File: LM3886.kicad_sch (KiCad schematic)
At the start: 1 part, among them U1 LM3886

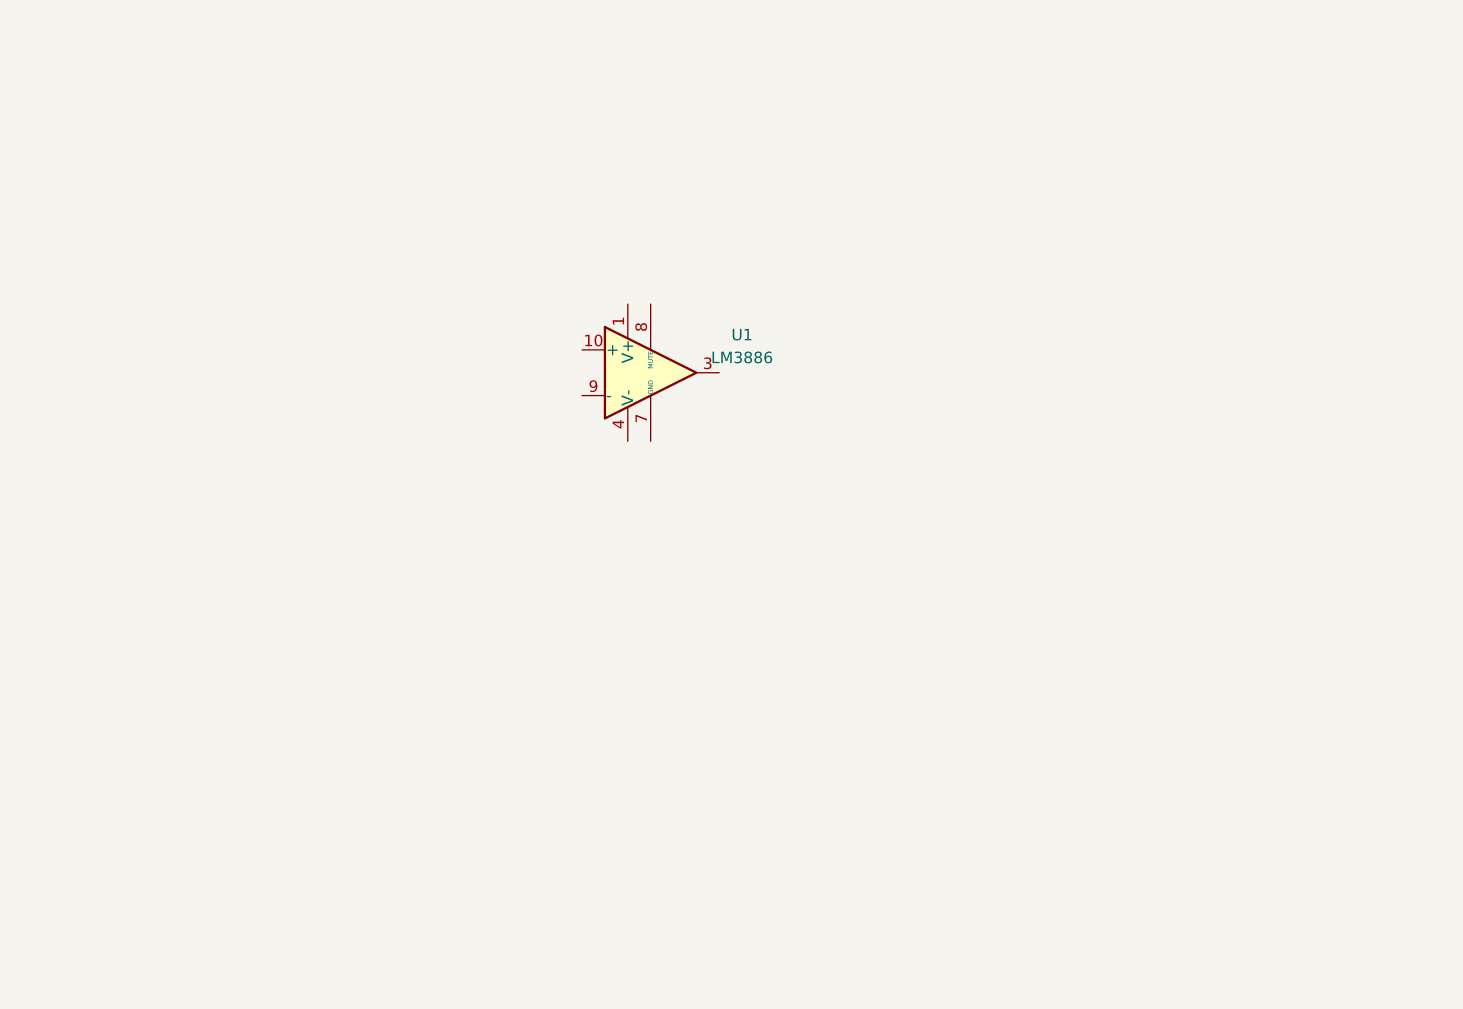
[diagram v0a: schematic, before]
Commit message: added schematic
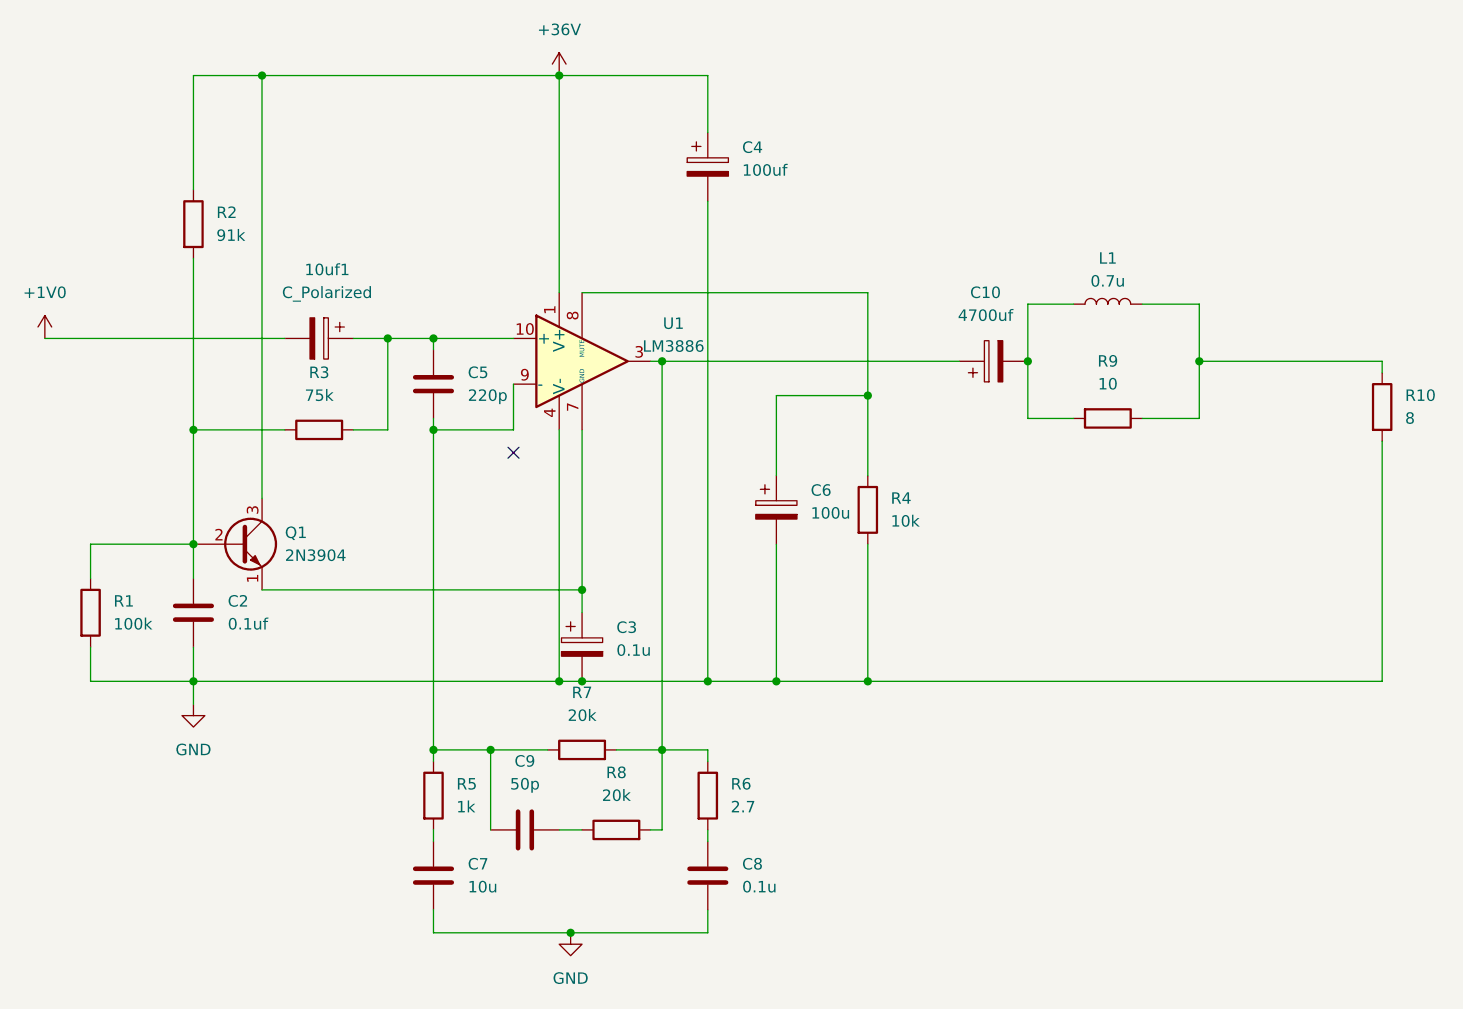
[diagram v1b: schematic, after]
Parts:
- added 10uf1: C_Polarized, Capacitor_THT:CP_Radial_Tantal_D4.5mm_P2.50mm, symbol Device:C_Polarized
- added C10: 4700uf, Capacitor_THT:CP_Radial_Tantal_D4.5mm_P2.50mm, symbol Device:C_Polarized
- added C2: 0.1uf, symbol Device:C
- added C3: 0.1u, Capacitor_THT:CP_Radial_Tantal_D4.5mm_P2.50mm, symbol Device:C_Polarized
- added C4: 100uf, Capacitor_THT:CP_Radial_Tantal_D4.5mm_P2.50mm, symbol Device:C_Polarized
- added C5: 220p, symbol Device:C
- added C6: 100u, Capacitor_THT:CP_Radial_Tantal_D4.5mm_P2.50mm, symbol Device:C_Polarized
- added C7: 10u, symbol Device:C
- added C8: 0.1u, symbol Device:C
- added C9: 50p, symbol Device:C
- added L1: 0.7u, symbol Device:L
- added Q1: 2N3904, Package_TO_SOT_THT:TO-92_Inline, symbol Transistor_BJT:2N3904
- added R1: 100k, symbol Device:R
- added R10: 8, symbol Device:R
- added R2: 91k, symbol Device:R
- added R3: 75k, symbol Device:R
- added R4: 10k, symbol Device:R
- added R5: 1k, symbol Device:R
- added R6: 2.7, symbol Device:R
- added R7, R8: 20k, symbol Device:R
- added R9: 10, symbol Device:R
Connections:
- net +36V: now reaches U1.1 (V+), U1.5 (V+)
- net +36V: now also C4.1, Q1.3 (C), R2.1
- net at U1.10 (+): now also 10uf1.1, C5.1, R3.2
- net at U1.3: now also C10.1, R6.1, R7.2, R8.2
- net GND: now reaches U1.4 (V-)
- net GND: now also C2.2, C3.2, C4.2, C6.2, C7.2, C8.2, R1.2, R10.2, R4.2
- net at U1.7 (GND): now also C3.1, Q1.1 (E)
- net at U1.8 (MUTE): now also C6.1, R4.1
- net at U1.9 (-): now also C5.2, C9.1, R5.1, R7.1
- new net: L1.2, R10.1, R9.1
- new net: C2.1, Q1.2 (B), R1.1, R2.2, R3.1
- new net: C7.1, R5.2
- new net: C10.2, L1.1, R9.2
- new net: C8.1, R6.2
- new net: C9.2, R8.1
- new net +1V0: 10uf1.2
- no-connect marks 0 -> 1
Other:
- moved on the sheet: U1
